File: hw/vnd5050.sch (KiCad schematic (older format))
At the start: 11 parts, among them U401 VND5050AJTR-E

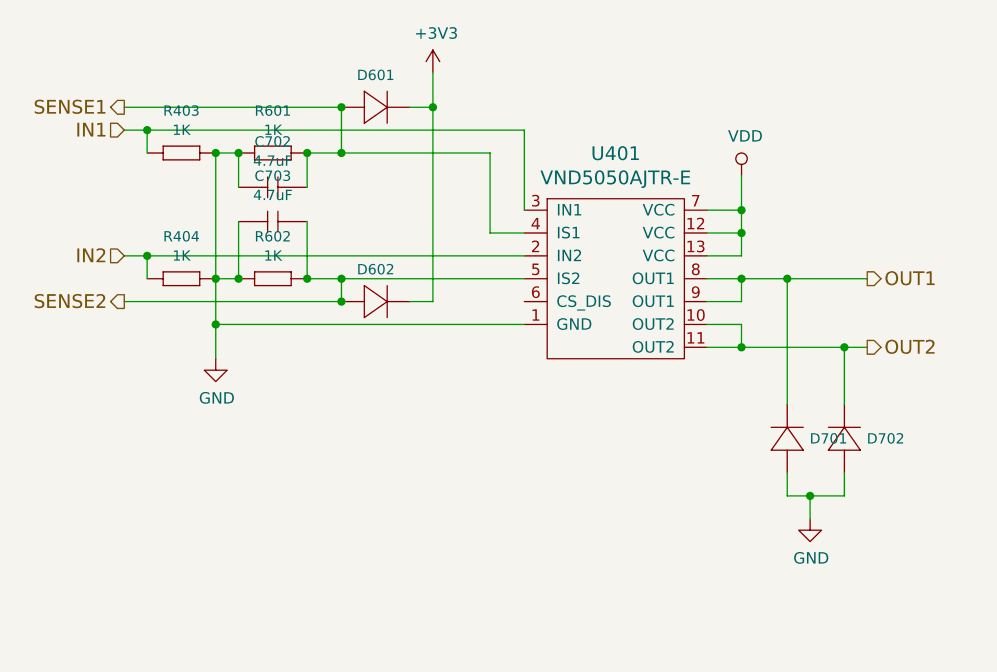
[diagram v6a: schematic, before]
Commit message: new ESB 5.2.0 sent
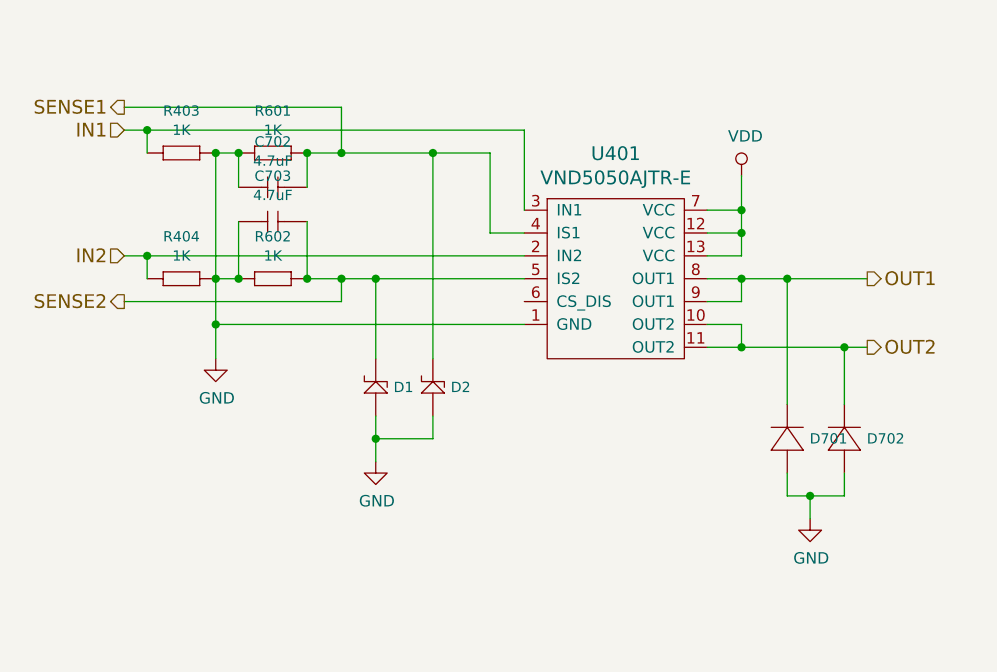
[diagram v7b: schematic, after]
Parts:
- removed D601, D602: DIODE_RS07J-GS18, usevolt:DO219AB, symbol usevolt:DIODE_RS07J-GS18
- added D1, D2: ZENER_MM3Z3V6T1G, usevolt:SOD-323, symbol usevolt:ZENER_MM3Z3V6T1G
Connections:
- net GND: now also D1.2, D2.2
- net SENSE1: now also D2.1
- net SENSE2: now also D1.1
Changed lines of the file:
@@
 $Descr A4 11693 8268
 encoding utf-8
-Sheet 6 12
+Sheet 6 13
 Title ""
 Date ""
@@
 	2950 4100 2950 4300
 Wire Wire Line
-	3500 4100 4300 4100
-Wire Wire Line
-	3500 3550 4150 3550
+	3500 4100 3650 4100
+Wire Wire Line
+	3500 3550 3900 3550
 Wire Wire Line
 	2650 3450 4300 3450
@@
 Connection ~ 3050 4100
 $Comp
-L usevolt:DIODE_RS07J-GS18 D602
-U 1 1 5B239934
-P 3700 4200
-F 0 "D602" H 3650 4340 45  0000 C CNN
-F 1 "DIODE_RS07J-GS18" H 3720 4140 45  0001 L BNN
-F 2 "usevolt:DO219AB" H 3730 4350 20  0001 C CNN
-F 3 "http://www.vishay.com/docs/85742/rs07b.pdf" H 3720 4220 60  0001 C CNN
-F 4 "1864882" H 4320 4820 60  0001 C CNN "2nd Source Part Number"
-F 5 "Digi-Key" H 4020 4520 60  0001 C CNN "1st Source"
-F 6 "Farnell" H 4220 4720 60  0001 C CNN "2nd Source"
-F 7 "RS07J-GS18" H 3920 4420 60  0001 C CNN "Manufacturer Part Number"
-F 8 "RS07J-GS18-ND" H 4120 4620 60  0001 C CNN "1st Source Part Number"
-F 9 "Vishay Semiconductor Diodes Division" H 3820 4320 60  0001 C CNN "Manufacturer"
-	1    3700 4200
-	1    0    0    -1
-$EndComp
-Connection ~ 3500 4200
-$Comp
-L usevolt:DIODE_RS07J-GS18 D601
-U 1 1 5B239A24
-P 3700 3350
-F 0 "D601" H 3650 3490 45  0000 C CNN
-F 1 "DIODE_RS07J-GS18" H 3720 3290 45  0001 L BNN
-F 2 "usevolt:DO219AB" H 3730 3500 20  0001 C CNN
-F 3 "http://www.vishay.com/docs/85742/rs07b.pdf" H 3720 3370 60  0001 C CNN
-F 4 "1864882" H 4320 3970 60  0001 C CNN "2nd Source Part Number"
-F 5 "Digi-Key" H 4020 3670 60  0001 C CNN "1st Source"
-F 6 "Farnell" H 4220 3870 60  0001 C CNN "2nd Source"
-F 7 "RS07J-GS18" H 3920 3570 60  0001 C CNN "Manufacturer Part Number"
-F 8 "RS07J-GS18-ND" H 4120 3770 60  0001 C CNN "1st Source Part Number"
-F 9 "Vishay Semiconductor Diodes Division" H 3820 3470 60  0001 C CNN "Manufacturer"
-	1    3700 3350
-	1    0    0    -1
-$EndComp
-Connection ~ 3500 3350
-$Comp
-L power:+3V3 #PWR0101
-U 1 1 5B239AE4
-P 3900 3200
-F 0 "#PWR0101" H 3900 3050 50  0001 C CNN
-F 1 "+3V3" H 3915 3373 50  0000 C CNN
-F 2 "" H 3900 3200 50  0000 C CNN
-F 3 "" H 3900 3200 50  0000 C CNN
-	1    3900 3200
-	1    0    0    -1
-$EndComp
-Wire Wire Line
-	3900 3200 3900 3350
-Wire Wire Line
-	3900 3350 3800 3350
-Wire Wire Line
-	3900 3350 3900 4200
-Wire Wire Line
-	3900 4200 3800 4200
-Connection ~ 3900 3350
+L usevolt:ZENER_MM3Z3V6T1G D1
+U 1 1 5BAA330C
+P 3650 4500
+F 0 "D1" V 3575 4422 45  0000 R CNN
+F 1 "ZENER_MM3Z3V6T1G" H 3925 4875 45  0001 L BNN
+F 2 "usevolt:SOD-323" H 3625 4875 20  0001 C CNN
+F 3 "http://www.mouser.com/ds/2/308/MM3Z2V4T1-D-269162.pdf" H 4000 5075 60  0001 C CNN
+F 4 "Mouser" H 3970 4820 60  0001 C CNN "1st Source"
+F 5 "MM3Z3V6T1G" H 3870 4720 60  0001 C CNN "Manufacturer Part Number"
+F 6 "863-MM3Z3V6T1G" H 4070 4920 60  0001 C CNN "1st Source Part Number"
+F 7 "ON Semiconductor" H 3925 4975 60  0001 C CNN "Manufacturer"
+	1    3650 4500
+	0    -1   -1   0
+$EndComp
+$Comp
+L usevolt:ZENER_MM3Z3V6T1G D2
+U 1 1 5BAA33EF
+P 3900 4500
+F 0 "D2" V 3825 4422 45  0000 R CNN
+F 1 "ZENER_MM3Z3V6T1G" H 4175 4875 45  0001 L BNN
+F 2 "usevolt:SOD-323" H 3875 4875 20  0001 C CNN
+F 3 "http://www.mouser.com/ds/2/308/MM3Z2V4T1-D-269162.pdf" H 4250 5075 60  0001 C CNN
+F 4 "Mouser" H 4220 4820 60  0001 C CNN "1st Source"
+F 5 "MM3Z3V6T1G" H 4120 4720 60  0001 C CNN "Manufacturer Part Number"
+F 6 "863-MM3Z3V6T1G" H 4320 4920 60  0001 C CNN "1st Source Part Number"
+F 7 "ON Semiconductor" H 4175 4975 60  0001 C CNN "Manufacturer"
+	1    3900 4500
+	0    -1   -1   0
+$EndComp
+Wire Wire Line
+	3900 4450 3900 3550
+Connection ~ 3900 3550
+Wire Wire Line
+	3900 3550 4150 3550
+Wire Wire Line
+	3650 4450 3650 4100
+Connection ~ 3650 4100
+Wire Wire Line
+	3650 4100 4300 4100
+$Comp
+L power:GND #PWR0101
+U 1 1 5BAA4BC4
+P 3650 4900
+F 0 "#PWR0101" H 3650 4650 50  0001 C CNN
+F 1 "GND" H 3655 4727 50  0000 C CNN
+F 2 "" H 3650 4900 50  0000 C CNN
+F 3 "" H 3650 4900 50  0000 C CNN
+	1    3650 4900
+	1    0    0    -1
+$EndComp
+Wire Wire Line
+	3650 4900 3650 4800
+Wire Wire Line
+	3650 4800 3900 4800
+Wire Wire Line
+	3900 4800 3900 4700
+Connection ~ 3650 4800
+Wire Wire Line
+	3650 4800 3650 4700
 $EndSCHEMATC
